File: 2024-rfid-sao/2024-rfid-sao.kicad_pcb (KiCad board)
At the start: 2 copper layers, 60 x 119.4 mm, 10 parts, among them U1 M24LR64E, X1 Badgelife_sao_connector_v169b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

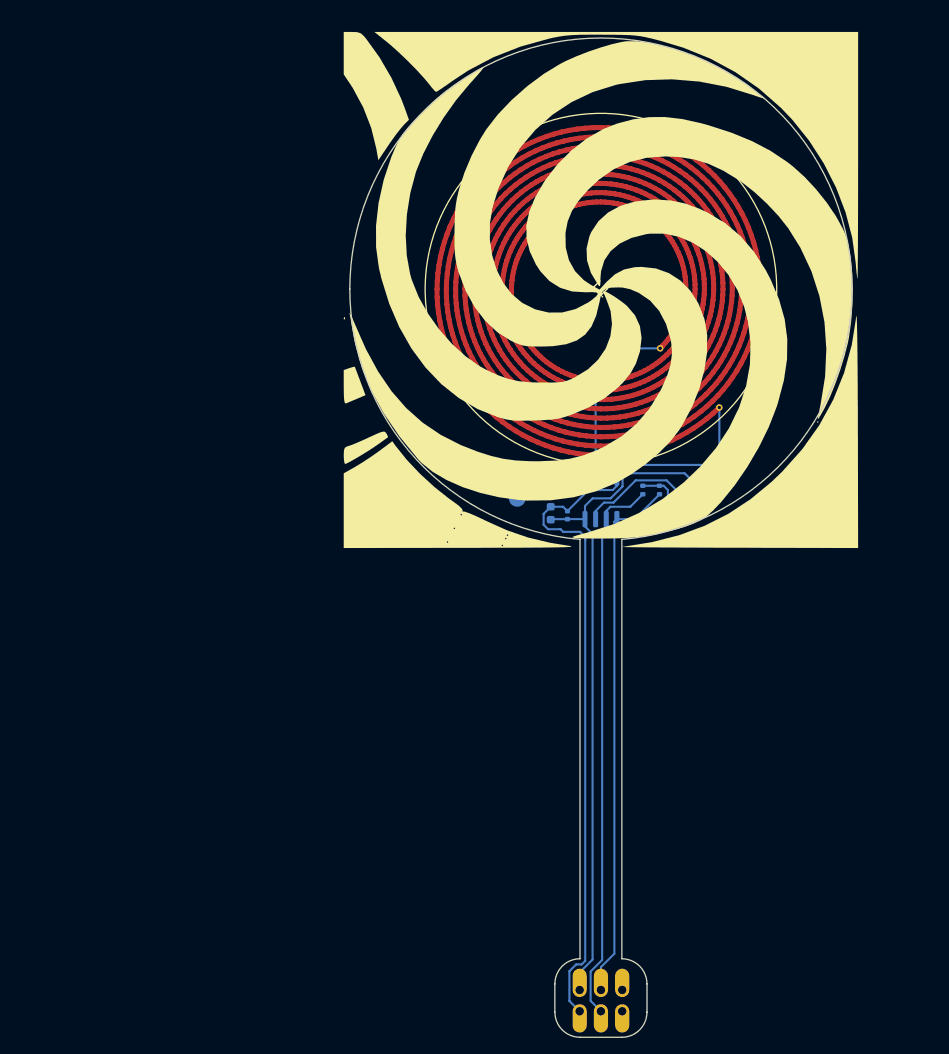
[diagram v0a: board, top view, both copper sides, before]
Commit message: 2024-rfid-sao: updates for jlcpcb
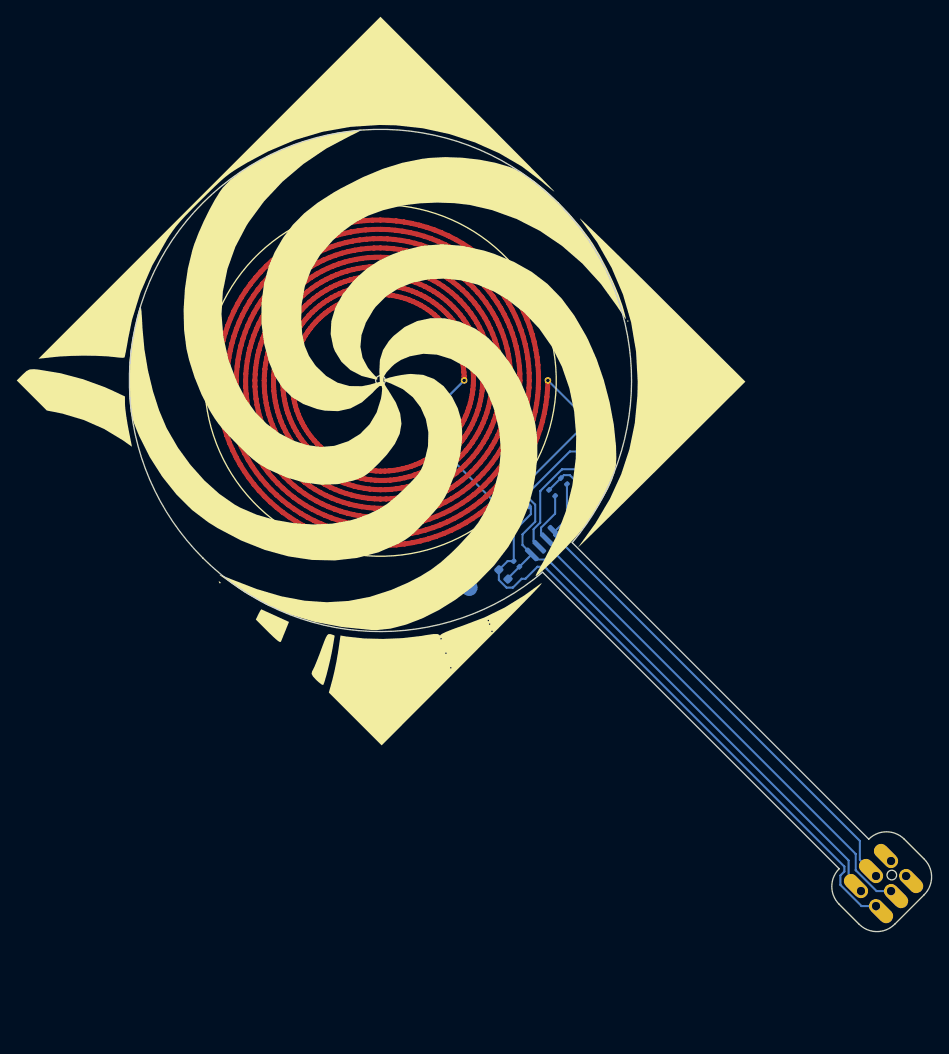
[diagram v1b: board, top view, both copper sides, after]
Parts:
- added REF**: JLC_TOOL_HOLE, library:JLC_TOOL_HOLE, F.Cu at (134.8, 170.0)
- added REF**: JLC_TOOL_HOLE, library:JLC_TOOL_HOLE, F.Cu at (73.7, 110.9)
- moved X1 36.5 mm to (133.8, 171.0), turned to -45 degrees
- moved G*** 28.5 mm to (73.7, 110.9), turned to 45 degrees
- moved L1 28.5 mm to (73.7, 110.9), turned to 0 degrees
- moved TP1 12.1 mm to (84.3, 135.7), turned to -135 degrees
- moved TP2 12.1 mm to (98.4, 121.5), turned to -135 degrees
- moved R2 11.5 mm to (95.6, 122.9), turned to -45 degrees
- moved R1 10.8 mm to (94.2, 124.3), turned to -45 degrees
- moved U1 9.38 mm to (91.3, 128.6), turned to -45 degrees
- moved C1 9.24 mm to (88.4, 134.1), turned to 135 degrees
- moved C2 8.42 mm to (89.9, 132.8), turned to 135 degrees
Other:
- board size 60 x 119.4 mm -> 95.8 x 95.8 mm
